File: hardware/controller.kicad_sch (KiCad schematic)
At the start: 83 parts, among them J1 USB_B_Micro, J10 Conn_01x06 Header, J11 Conn_01x04 MiniPV, J16 Conn_01x03 MiniPV, J2 Conn_01x04 Header, J3 Conn_01x02 MiniPV, J4 Conn_01x02 MiniPV, J5 Conn_01x03 MiniPV, J6 Conn_01x03 MiniPV, J7 Conn_01x03 MiniPV, J8 Conn_01x03 MiniPV, J9 Conn_01x03 MiniPV, Q1 AO3400A, Q2 AO3400A, Q3 AO3400A, Q4 AO3400A, Q7 AO3400A, SW1 SW_Push, U1 STM32G030C8T6, U2 CH340C, U3 MAX31855KASA, U4 MAX31855KASA

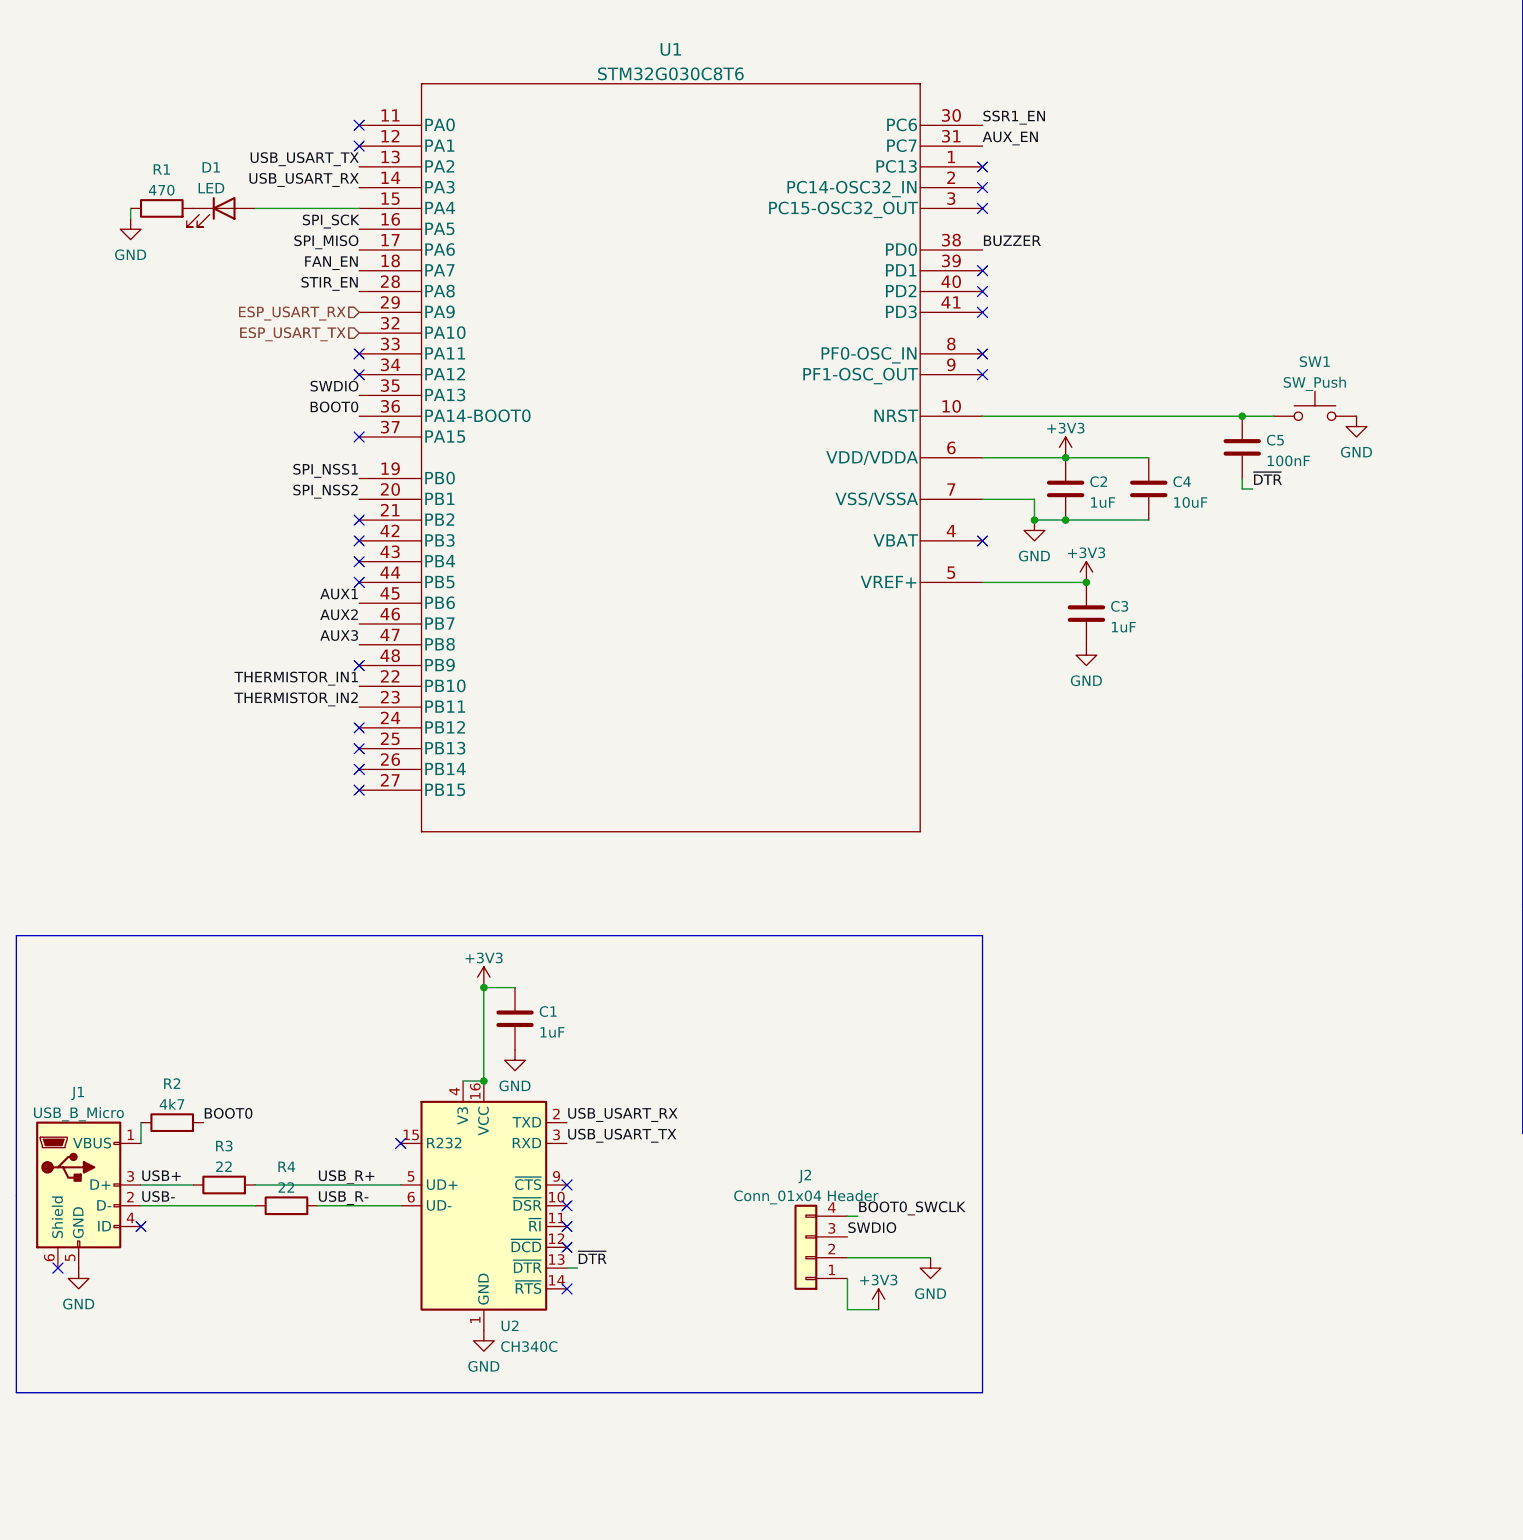
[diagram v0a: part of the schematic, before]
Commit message: Continue layout
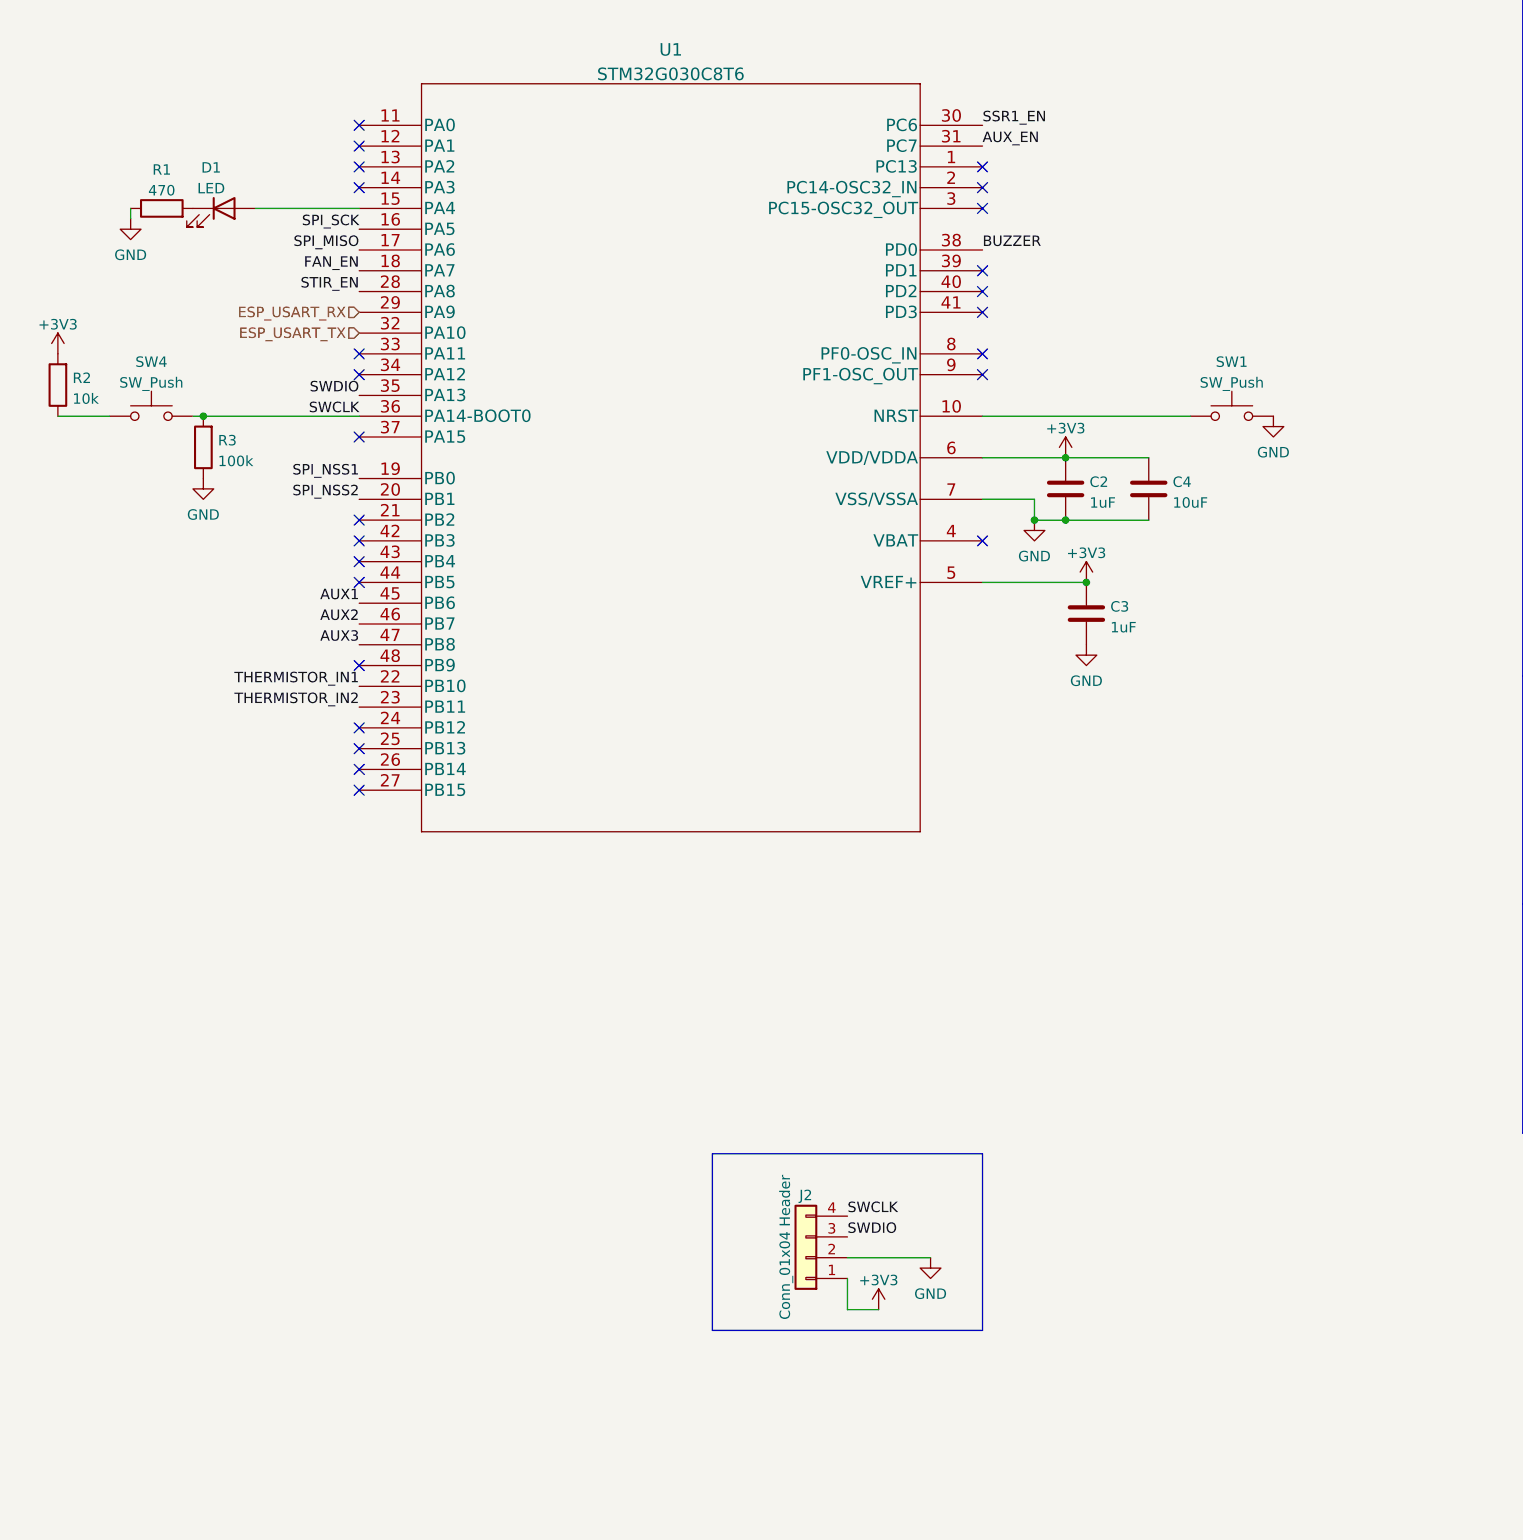
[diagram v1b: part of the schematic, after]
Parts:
- removed C1: 1uF, Capacitor_SMD:C_0402_1005Metric, symbol Device:C
- removed C5: 100nF, Capacitor_SMD:C_0402_1005Metric, symbol Device:C
- removed J1: USB_B_Micro, Homebrew:FRAMATOME_10118194-0001LF_fixed_bridges, symbol Connector:USB_B_Micro
- removed R4: 22, Resistor_SMD:R_0402_1005Metric, symbol Device:R
- removed U2: CH340C, Package_SO:SOIC-16_3.9x9.9mm_P1.27mm, symbol Interface_USB:CH340C
- added SW4: SW_Push, Homebrew:SW_TACTILE_5.1MM_TS-1187A-C-D-B, symbol Switch:SW_Push
- R2: value 4k7 -> 10k; LCSC C25900 -> C25744
- R3: value 22 -> 100k; LCSC C25091 -> C25741
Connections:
- net BOOT0_SWCLK is gone; now on net SWCLK: J2.4 (Pin_4)
- net USB+ is gone; now on net GND: R3.1
- net USB_R+ is gone; now on net SWCLK: R3.2
- net +3V3: now also R2.2
- net at R2.1: now also SW4.1
- net BOOT0 renamed SWCLK
- net SWCLK: now also SW4.2; no longer R2.2
- net USB_USART_RX: no longer names the net of U1.14 (PA3)
- net USB_USART_TX: no longer names the net of U1.13 (PA2)
- no-connect marks 36 -> 30
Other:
- moved on the sheet: SW1
